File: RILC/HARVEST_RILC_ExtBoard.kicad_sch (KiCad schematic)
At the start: 47 parts, among them J3 Conn_01x02, SW1 SW_SPST, SW2 SW_DIP_x04, U1 TPS92612DBVR, U2 TPS92612DBVR, U3 TPS92612DBVR, U4 TPS92612DBVR

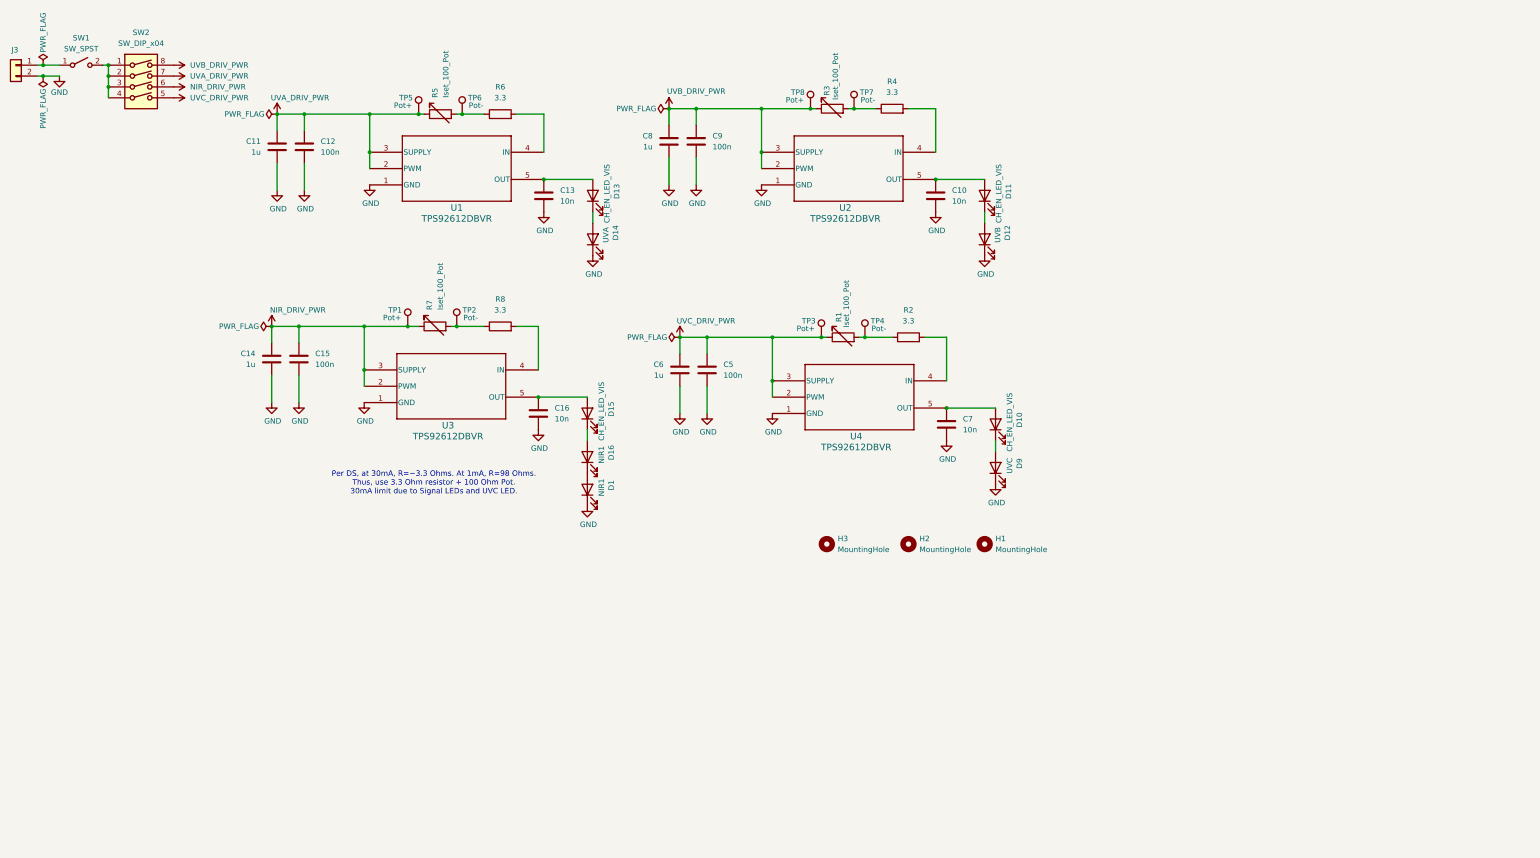
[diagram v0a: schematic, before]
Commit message: V2.0: Produced Version
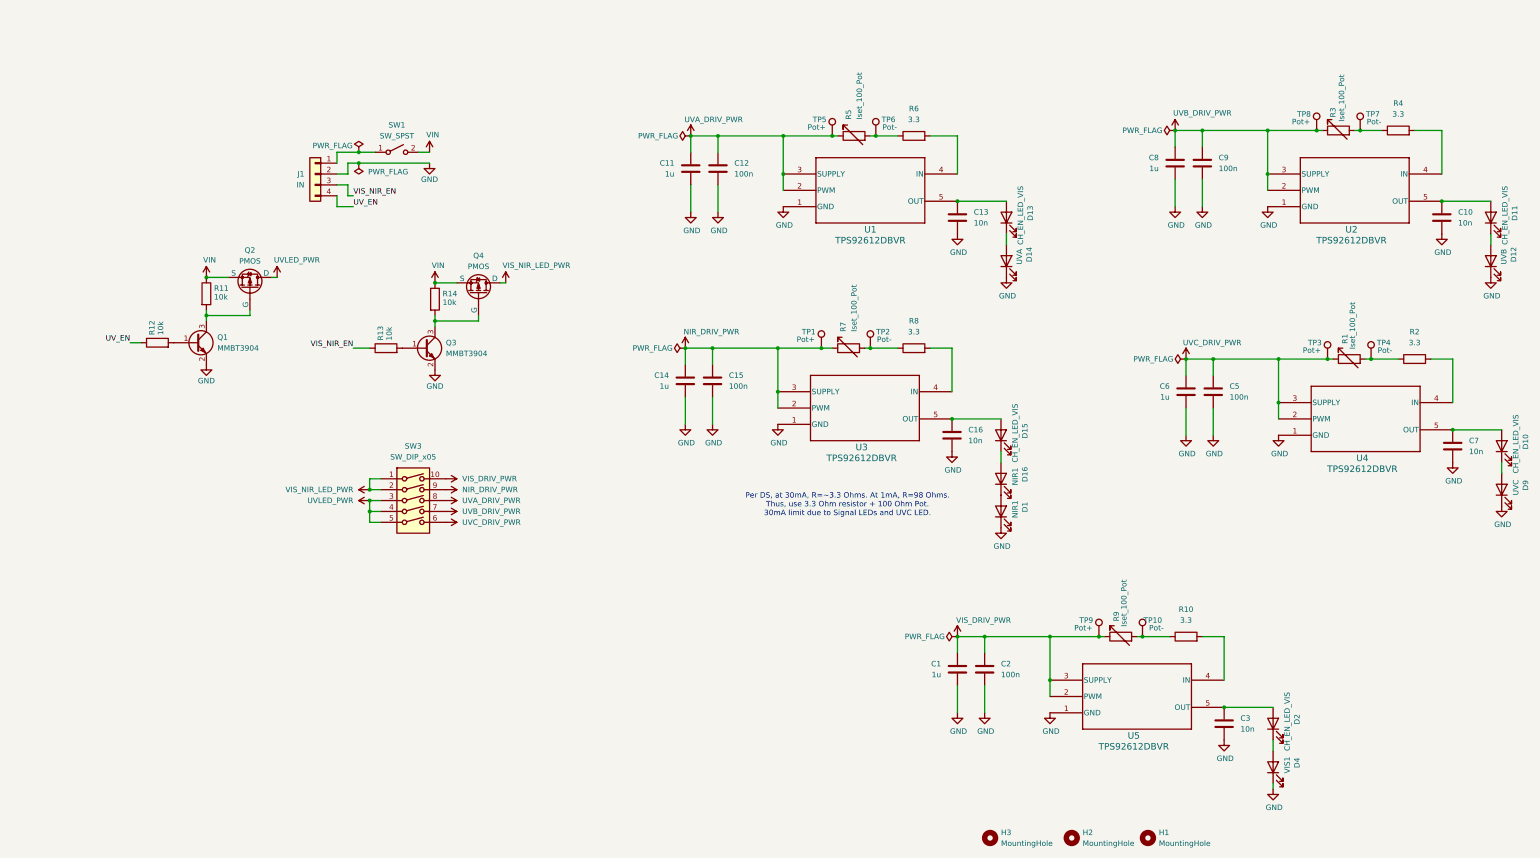
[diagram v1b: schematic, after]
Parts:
- removed J3: Conn_01x02, Connector_JST:JST_XH_B2B-XH-A_1x02_P2.50mm_Vertical, symbol Connector_Generic:Conn_01x02
- removed SW2: SW_DIP_x04, Button_Switch_THT:SW_DIP_SPSTx04_Piano_CTS_Series194-4MSTN_W7.62mm_P2.54mm, symbol Switch:SW_DIP_x04
- added C1: 1u, Capacitor_SMD:C_0805_2012Metric_Pad1.18x1.45mm_HandSolder, symbol Device:C
- added C2: 100n, Capacitor_SMD:C_0805_2012Metric_Pad1.18x1.45mm_HandSolder, symbol Device:C
- added C3: 10n, Capacitor_SMD:C_0805_2012Metric_Pad1.18x1.45mm_HandSolder, symbol Device:C
- added D2: CH_EN_LED_VIS, LED_SMD:LED_0805_2012Metric_Pad1.15x1.40mm_HandSolder, symbol Device:LED
- added D4: VIS1, 158301240_LED:WL-SWTP_3014, symbol Device:LED
- added J1: IN, Connector_JST:JST_XH_B4B-XH-A_1x04_P2.50mm_Vertical, symbol Connector_Generic:Conn_01x04
- added Q1, Q3: MMBT3904, Package_TO_SOT_SMD:SOT-23, symbol Transistor_BJT:MMBT3904
- added Q2, Q4: PMOS, DMG2305UX-7_Snapeda:SOT91P240X110-3N_DMG2305UX-7, symbol Simulation_SPICE:PMOS
- added R10: 3.3, Resistor_SMD:R_0805_2012Metric_Pad1.20x1.40mm_HandSolder, symbol Device:R
- added R11, R12, R13, R14: 10k, Resistor_SMD:R_0805_2012Metric_Pad1.20x1.40mm_HandSolder, symbol Device:R
- added R9: Iset_100_Pot, Potentiometer_THT:Potentiometer_Bourns_3296W_Vertical, symbol Device:R_Variable
- added SW3: SW_DIP_x05, Button_Switch_THT:SW_DIP_SPSTx05_Piano_CTS_Series194-5MSTN_W7.62mm_P2.54mm, symbol Switch:SW_DIP_x05
- added TP10: Pot-, TestPoint:TestPoint_Pad_1.5x1.5mm, symbol Connector:TestPoint
- added TP9: Pot+, TestPoint:TestPoint_Pad_1.5x1.5mm, symbol Connector:TestPoint
- added U5: TPS92612DBVR, TPS92612:SOT_12DBVR_TEX, symbol TPS29612:TPS92612DBVR
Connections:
- net GND: now also C1.2, C2.2, C3.2, D4.1 (K), J1.2 (Pin_2), Q1.2 (E), Q3.2 (E), U5.1 (GND)
- net NIR_DRIV_PWR: now also SW3.9
- net UVA_DRIV_PWR: now also SW3.8
- net UVB_DRIV_PWR: now also SW3.7
- net UVC_DRIV_PWR: now also SW3.6
- net at SW1.1 (A): now also J1.1 (Pin_1)
- net VIN: now reaches SW1.2 (B)
- net VIN: now also Q2.3 (S), Q4.3 (S), R11.1, R14.1
- new net: Q1.1 (B), R12.2
- new net: Q1.3 (C), Q2.2 (G), R11.2
- new net: D2.1 (K), D4.2 (A)
- new net: C3.1, D2.2 (A), U5.5 (OUT)
- new net: R10.1, R9.2, TP10.1
- new net: R10.2, U5.4 (IN)
- new net: Q3.3 (C), Q4.2 (G), R14.2
- new net: Q3.1 (B), R13.2
- new net UVLED_PWR: Q2.1 (D), SW3.3, SW3.4, SW3.5
- new net UV_EN: J1.4 (Pin_4), R12.1
- new net VIS_DRIV_PWR: C1.1, C2.1, R9.1, SW3.10, TP9.1, U5.2 (PWM), U5.3 (SUPPLY)
- new net VIS_NIR_EN: J1.3 (Pin_3), R13.1
- new net VIS_NIR_LED_PWR: Q4.1 (D), SW3.1, SW3.2
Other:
- moved on the sheet: C10, C11, C12, C13, C14, C15, C16, C5, C6, C7, C8, C9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
